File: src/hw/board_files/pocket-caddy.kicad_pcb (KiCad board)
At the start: 4 copper layers, 92 parts, among them J1 Test_Points, J2 Conn_01x03_Pin, J3 Conn_01x03_Pin, J4 MSD-1-A, P1 USB_C_Plug_USB2.0, Q1 PMOS, SW1 SW_PWR, SW2 RESET, SW3 BTN_1_BOOT, SW4 BTN_2, SW5 BTN_3, U1 TPS63031DSKR, U2 FT234XD-R, U3 MCP73871, U4 ESP32-C3-WROOM-02, U5 SHT30-DIS, U6 NEO-M9N, U7 BQ27427, U8 NHD-C0220BIZ-FSRGB, Y1 32.768kHz

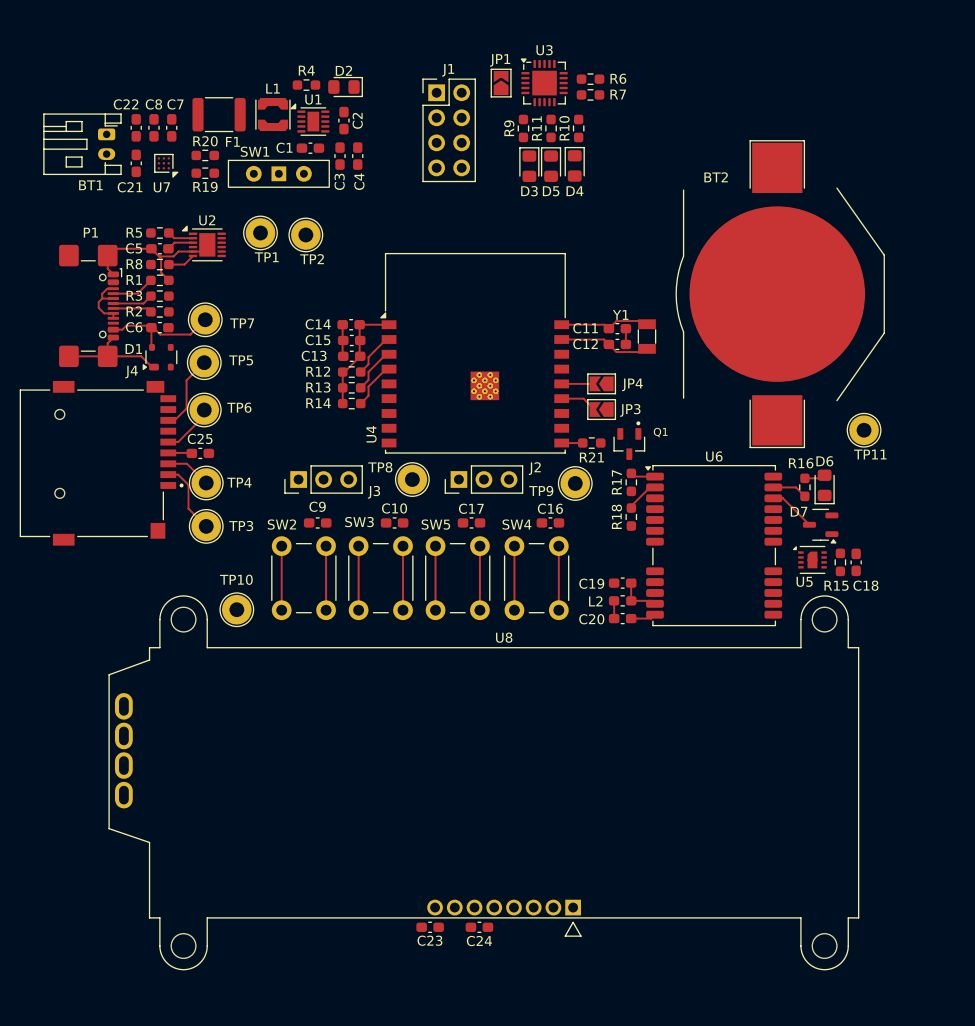
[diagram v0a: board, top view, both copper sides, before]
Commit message: Started working on layout traces
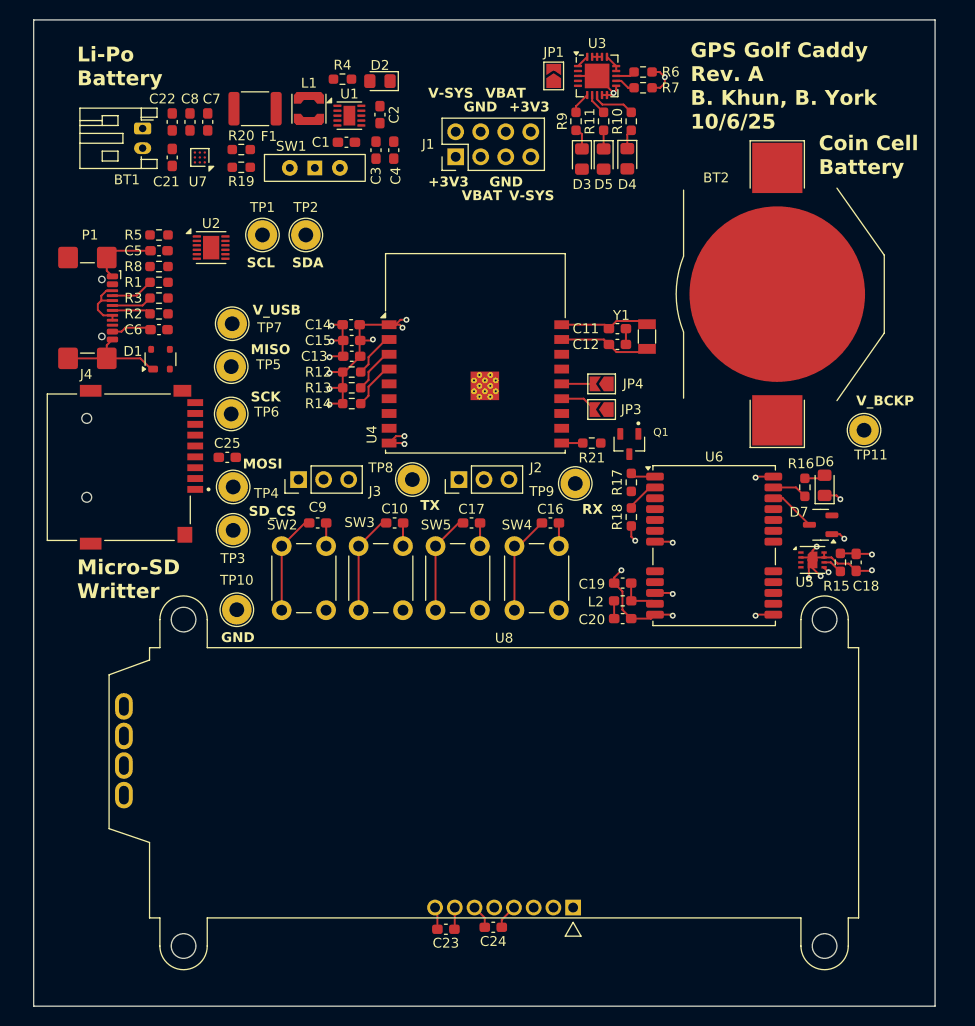
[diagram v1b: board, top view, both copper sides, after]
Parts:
- moved J1 6.78 mm to (73.8, 52.1), turned to 90 degrees
- moved R9 5.38 mm to (86.0, 48.5)
- moved D3 5.38 mm to (86.6, 52.3)
- moved D4 5.38 mm to (91.2, 52.3)
- moved D5 5.38 mm to (88.8, 52.3)
- moved JP1 5.38 mm to (83.7, 43.9)
- moved R10 5.38 mm to (91.6, 48.5)
- moved R11 5.38 mm to (88.8, 48.5)
- moved R6 5.38 mm to (92.8, 43.5)
- moved U3 5.38 mm to (88.1, 43.9)
- moved R7 5.38 mm to (92.8, 45.1)
- moved C3 3.70 mm to (65.7, 51.4)
- moved C4 3.70 mm to (67.5, 51.4)
- moved U1 3.70 mm to (63.0, 47.9)
- moved F1 3.70 mm to (53.5, 47.2)
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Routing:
- net GND: track 61.5 -> 86.4 mm, vias 0 -> 18
- net +3V3: track 14.3 -> 27.9 mm, vias 0 -> 10
- net /SD_CS: track 9.57 -> 2.14 mm
- net V_USB: track 12.7 -> 5.31 mm
- net /SPI_MISO: track 7.74 -> 0.65 mm
- net /SPI_SCK: track 5.35 -> 0.60 mm
- net /SPI_MOSI: track 4.66 -> 0.00 mm
- net Net-(U3-STAT1/~{LBO}): track 0.00 -> 4.44 mm
- net Net-(U4-EN): track 11.2 -> 14.9 mm
- net /Microcontroller/BTN_3: track 6.50 -> 10.3 mm
- net /Microcontroller/BTN_2: track 6.50 -> 10.3 mm
- net /Microcontroller/BTN_1_BOOT: track 6.50 -> 10.3 mm
- net Net-(U2-CBUS0): track 2.81 -> 0.00 mm
- net Net-(U2-3V3OUT): track 2.75 -> 0.00 mm
- net Net-(U2-~{RESET}): track 2.67 -> 0.00 mm
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- added copper zone on In1.Cu, net +3V3
- added copper zone on In2.Cu, net GND
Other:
- board outline added: 91.4 x 100 mm
- board text added: "+3V3"
- board text added: "Coin Cell Battery"
- board text added: "GND"
- board text added: "GPS Golf Caddy Rev. A B. Khun, B. York 10/6/25"
- board text added: "Li-Po Battery"
- board text added: "MISO"
- board text added: "MOSI"
- board text added: "Micro-SD Writter"
- board text added: "RX"
- board text added: "SCK"
- board text added: "SCL"
- board text added: "SDA"
- board text added: "SD_CS"
- board text added: "TX"
- board text added: "V-SYS"
- board text added: "VBAT"
- board text added: "V_BCKP"
- board text added: "V_USB"
- board text removed: "Antenna"
- board text removed: "LCD CONNECTOR"
